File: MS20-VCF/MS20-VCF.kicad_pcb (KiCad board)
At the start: 2 copper layers, 127.5 x 133 mm, 112 parts, among them J1 Conn_CircuitBoard, J10 Conn_CircuitBoard, J11 Conn_JackBoard, J12 Conn_JackBoard, J13 FilterCV2, J14 FilterIn2, J15 FilterOut2, J2 Conn_CircuitBoard, J3 Conn_JackBoard, J4 Conn_JackBoard, J5 Power Input, J6 FilterCV1, J7 FilterIn1, J8 FilterOut1, J9 Conn_CircuitBoard, Q1 BC559, Q2 BC559, Q3 BC559, Q4 BC559, SW1 Hpass/Lpass Switch, SW2 Bandpass, SW3 Hpass/Lpass Switch, U1 LM13700, U2 TL072, U3 LM13700, U4 TL072

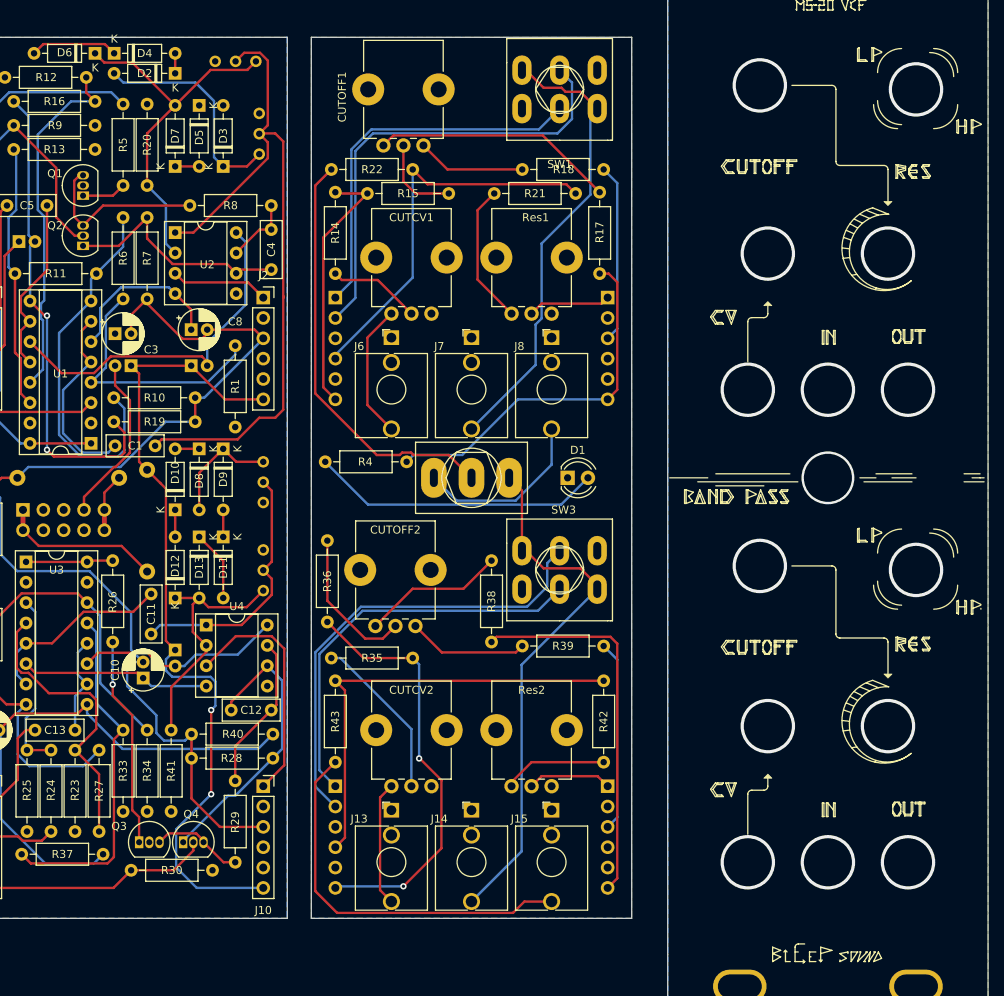
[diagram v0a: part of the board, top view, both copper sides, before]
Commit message: updgrade MS20
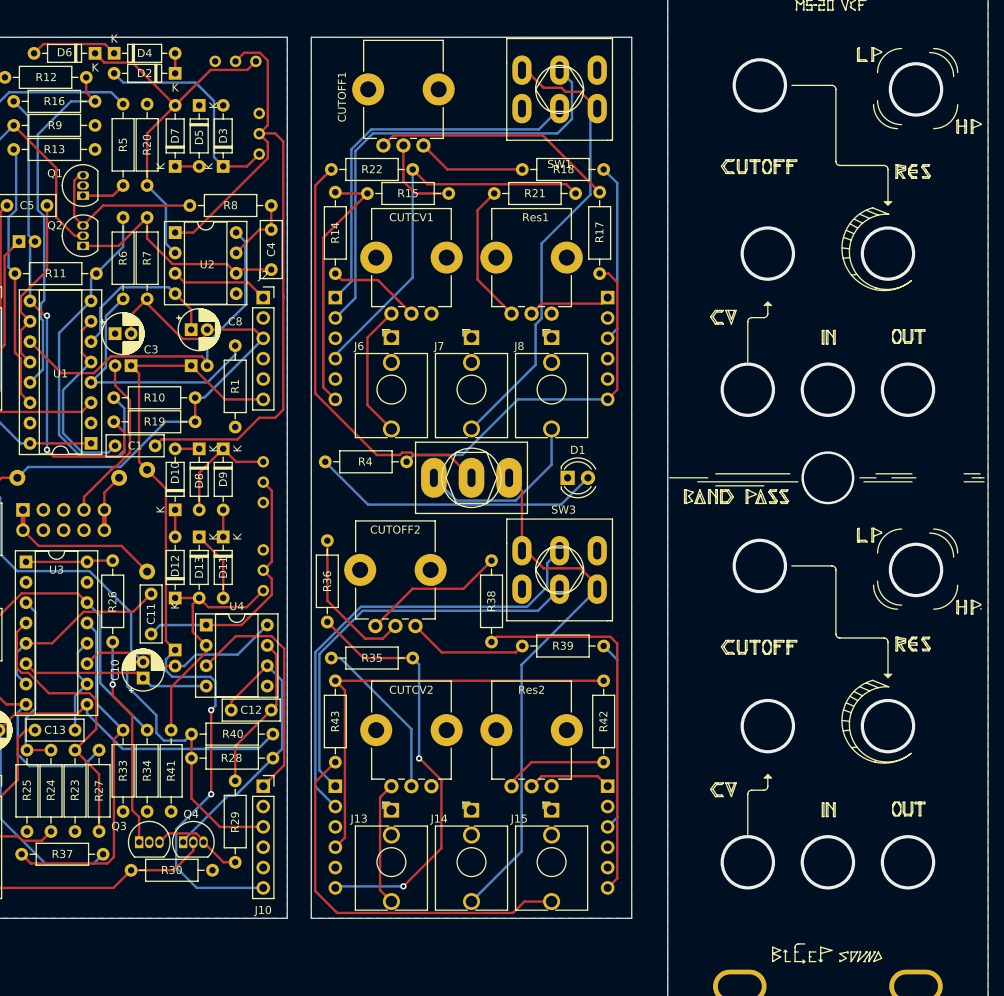
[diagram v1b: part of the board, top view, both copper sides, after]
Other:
- net class Default removed
- net class Power removed

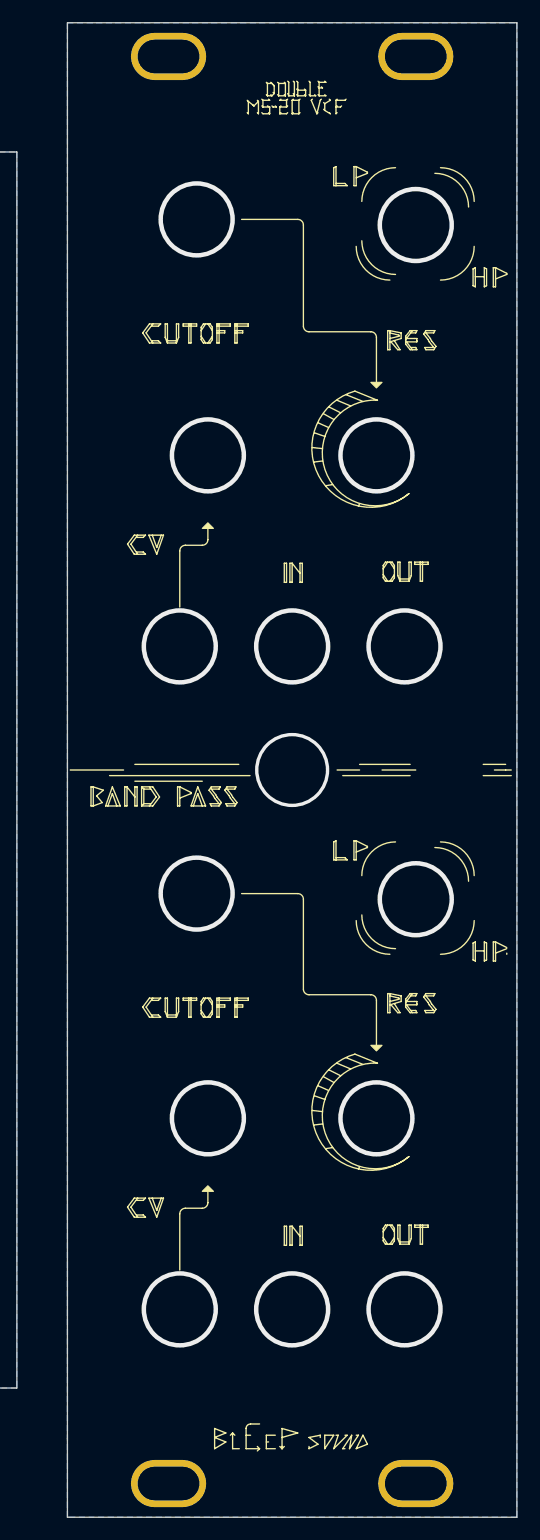
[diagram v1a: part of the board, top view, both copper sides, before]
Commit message: Update gerber MS20-VCF
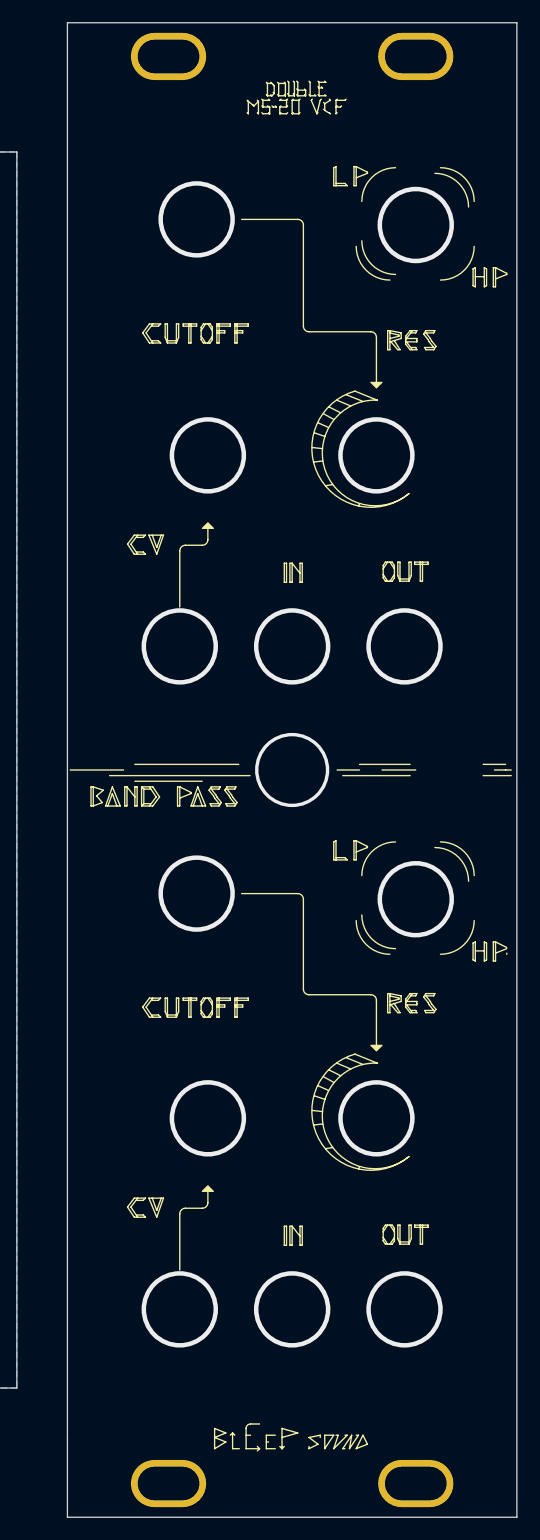
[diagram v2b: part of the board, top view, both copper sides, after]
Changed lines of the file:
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@@
     (fp_line (start 4 -2.75) (end -1.45 -2.75) (layer "F.CrtYd") (width 0.05))
     (fp_line (start -0.73 -1.32665) (end -0.73 1.32665) (layer "F.Fab") (width 0.1))
-    (fp_arc (start -0.73 -1.32665) (mid 3.67 0.000306) (end -0.730339 1.32614) (layer "F.Fab") (width 0.1))
+    (fp_arc (start -0.73 -1.32665) (mid 3.670001 0.000308) (end -0.730339 1.32614) (layer "F.Fab") (width 0.1))
     (fp_circle (center 1.27 0) (end 3.27 0) (layer "F.Fab") (width 0.1) (fill none))
     (pad "1" thru_hole rect locked (at 0 0) (size 1.8 1.8) (drill 0.9) (layers *.Cu *.Mask)
@@
   (gr_line (start 140.7 61) (end 139.8 60.6) (layer "F.SilkS") (width 0.12))
   (gr_arc (start 147.880994 66.91004) (mid 140.425465 64.78058) (end 145.085033 58.583166) (layer "F.SilkS") (width 0.12))
-  (gr_arc (start 147.9 66.9) (mid 139.860984 65.315822) (end 143.085033 57.783166) (layer "F.SilkS") (width 0.12))
+  (gr_arc (start 147.9 66.9) (mid 139.860985 65.315822) (end 143.085033 57.783166) (layer "F.SilkS") (width 0.12))
   (gr_line (start 143.8 58.7) (end 142.3 58.1) (layer "F.SilkS") (width 0.12))
   (gr_arc (start 130 71) (mid 129.853553 71.353553) (end 129.5 71.5) (layer "F.SilkS") (width 0.12))
@@
   (gr_line (start 141.2 119.3) (end 140.3 118.8) (layer "F.SilkS") (width 0.12))
   (gr_line (start 140.414967 120.816834) (end 139.5 120.5) (layer "F.SilkS") (width 0.12))
-  (gr_arc (start 147.9 125.9) (mid 139.860984 124.315822) (end 143.085033 116.783166) (layer "F.SilkS") (width 0.12))
+  (gr_arc (start 147.9 125.9) (mid 139.860985 124.315822) (end 143.085033 116.783166) (layer "F.SilkS") (width 0.12))
   (gr_line (start 140.2 121.9) (end 139.3 121.8) (layer "F.SilkS") (width 0.12))
   (gr_line (start 139.4 123.1) (end 140.2 123) (layer "F.SilkS") (width 0.12))
@@
   (gr_line (start 137.5 139.5) (end 137.5 133.7) (layer "Dwgs.User") (width 0.15))
   (gr_line (start 147.5 139.5) (end 147.5 133.5) (layer "Dwgs.User") (width 0.15))
-  (gr_line (start 129 42.5) (end 84.5 42.5) (layer "Dwgs.User") (width 0.15))
   (gr_line (start 113 95) (end 73 95) (layer "Dwgs.User") (width 0.15))
   (gr_line (start 69.999999 36.5) (end 70 146.5) (layer "Edge.Cuts") (width 0.05))
@@
   (segment (start 49.257997 67.700001) (end 46.650001 70.307997) (width 0.3) (layer "B.Cu") (net 15))
   (segment (start 54.202002 115) (end 52.552001 113.349999) (width 0.3) (layer "F.Cu") (net 16))
+  (segment (start 46.350001 113.349999) (end 45 114.7) (width 0.3) (layer "F.Cu") (net 16))
   (segment (start 52.552001 113.349999) (end 46.350001 113.349999) (width 0.3) (layer "F.Cu") (net 16))
   (segment (start 56 115) (end 54.202002 115) (width 0.3) (layer "F.Cu") (net 16))
-  (segment (start 46.350001 113.349999) (end 45 114.7) (width 0.3) (layer "F.Cu") (net 16))
   (segment (start 45.350001 114.349999) (end 45 114.7) (width 0.3) (layer "B.Cu") (net 16))
   (segment (start 63.809999 113.570001) (end 58.561369 113.570001) (width 0.3) (layer "B.Cu") (net 16))
@@
   (zone (net 1) (net_name "GND") (layer "B.Cu") (hatch edge 0.508)
     (connect_pads (clearance 0.508))
-    (min_thickness 0.254)
+    (min_thickness 0.254) (filled_areas_thickness no)
     (fill yes (thermal_gap 0.508) (thermal_bridge_width 0.508))
     (polygon
@@
   (zone (net 1) (net_name "GND") (layer "B.Cu") (hatch edge 0.508)
     (connect_pads (clearance 0.508))
-    (min_thickness 0.254)
+    (min_thickness 0.254) (filled_areas_thickness no)
     (fill yes (thermal_gap 0.508) (thermal_bridge_width 0.508))
     (polygon
@@
       )
     )
-  )
-  (zone (net 1) (net_name "GND") (layer "B.Cu") (hatch edge 0.508)
-    (connect_pads (clearance 0.508))
-    (min_thickness 0.254)
-    (fill yes (thermal_gap 0.508) (thermal_bridge_width 0.508))
-    (polygon
-      (pts
-        (xy 157.5 158)
-        (xy 117.5 158)
-        (xy 117.5 25)
-        (xy 157.5 25)
-      )
-    )

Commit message: update MS-20 VCF (increase size)
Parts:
- added C15: 0.1µ, Capacitor_THT:CP_Radial_D5.0mm_P2.00mm, F.Cu at (34.0, 107.5)
- added C16: 0.1µ, Capacitor_THT:CP_Radial_D5.0mm_P2.00mm, F.Cu at (34.0, 103.5)
- added C17: 0.1µ, Capacitor_THT:CP_Radial_D5.0mm_P2.00mm, F.Cu at (34.0, 91.5)
- added C18: 0.1µ, Capacitor_THT:CP_Radial_D5.0mm_P2.00mm, F.Cu at (37.0, 98.0)
- C2, C6, C7, C9: moved to F.Cu
- moved H2 79.5 mm to (228.0, 29.5)
- moved H3 79.5 mm to (228.0, 153.5)
- moved R4 64.5 mm to (147.0, 71.9), turned to -90 degrees
- moved H1 59.5 mm to (186.0, 29.5)
- moved H4 59.5 mm to (186.0, 153.5)
- moved R38 57.8 mm to (152.0, 113.9)
- moved R22 56.9 mm to (130.1, 69.0), turned to 180 degrees
- moved CUTOFF2 56.5 mm to (142.5, 110.0)
- moved CUTCV1 52.5 mm to (140.5, 71.0)
- moved J6 52.0 mm to (135.0, 74.0)
- moved D1 43.6 mm to (148.3, 86.5), turned to 180 degrees
- moved R9 43.0 mm to (74.1, 80.0)
- moved J12 42.0 mm to (152.0, 130.0)
- moved J4 42.0 mm to (152.0, 69.0)
- moved R39 40.2 mm to (148.0, 124.1), turned to 90 degrees
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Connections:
- C7 pad 2: Net-(C7-Pad2) -> Net-(U2-Pad8)
- J1 pad 3: Net-(J1-Pad3) -> unconnected-(J1-Pad3)
- J1 pad 5: Net-(J1-Pad5) -> unconnected-(J1-Pad5)
- J10 pad 2: Net-(J10-Pad2) -> unconnected-(J10-Pad2)
- J11 pad 3: Net-(J11-Pad3) -> unconnected-(J11-Pad3)
- J11 pad 5: Net-(J11-Pad5) -> unconnected-(J11-Pad5)
- J12 pad 2: Net-(J12-Pad2) -> unconnected-(J12-Pad2)
- J13 pad TN: Net-(J13-PadTN) -> unconnected-(J13-PadTN)
- J14 pad TN: Net-(J14-PadTN) -> unconnected-(J14-PadTN)
- J15 pad TN: Net-(J15-PadTN) -> unconnected-(J15-PadTN)
- J2 pad 2: Net-(J2-Pad2) -> unconnected-(J2-Pad2)
- J3 pad 3: Net-(J3-Pad3) -> unconnected-(J3-Pad3)
- J3 pad 5: Net-(J3-Pad5) -> unconnected-(J3-Pad5)
- J4 pad 2: Net-(J4-Pad2) -> unconnected-(J4-Pad2)
- J6 pad TN: Net-(J6-PadTN) -> unconnected-(J6-PadTN)
- J7 pad TN: Net-(J7-PadTN) -> unconnected-(J7-PadTN)
- J8 pad TN: Net-(J8-PadTN) -> unconnected-(J8-PadTN)
- J9 pad 3: Net-(J9-Pad3) -> unconnected-(J9-Pad3)
- J9 pad 5: Net-(J9-Pad5) -> unconnected-(J9-Pad5)
- SW1 pad 1: Net-(SW1-Pad1) -> unconnected-(SW1-Pad1)
- SW3 pad 1: Net-(SW3-Pad1) -> unconnected-(SW3-Pad1)
- U1 pad 11: Net-(C7-Pad2) -> Net-(U1-Pad11)
- U1 pad 15: Net-(U1-Pad15) -> unconnected-(U1-Pad15)
- U1 pad 2: Net-(U1-Pad2) -> unconnected-(U1-Pad2)
- U1 pad 6: Net-(C8-Pad1) -> Net-(C18-Pad1)
- U2 pad 8: Net-(C7-Pad2) -> Net-(U2-Pad8)
- U3 pad 11: Net-(C9-Pad2) -> Net-(C15-Pad2)
- U3 pad 15: Net-(U3-Pad15) -> unconnected-(U3-Pad15)
- U3 pad 2: Net-(U3-Pad2) -> unconnected-(U3-Pad2)
- U3 pad 6: Net-(C10-Pad1) -> Net-(C16-Pad1)
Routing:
- net Net-(R5-Pad2): track 71.7 -> 13.4 mm
- net Net-(C7-Pad2): track 44.5 -> 0.00 mm
- net /ResOut: track 22.6 -> 57.4 mm, vias 0 -> 1
- net -12V: track 183.6 -> 218.2 mm, vias 0 -> 1
- net Net-(C18-Pad1): track 0.00 -> 34.1 mm, vias 0 -> 1
- net Net-(C14-Pad2): track 66.0 -> 32.3 mm
- net Net-(C1-Pad2): track 88.4 -> 54.8 mm
- net Net-(D1-Pad2): track 36.4 -> 4.94 mm
- net Net-(R2-Pad2): track 45.7 -> 16.2 mm
- net Net-(CUTOFF2-Pad2): track 18.6 -> 47.4 mm
- net +12V: track 196.4 -> 225.1 mm, vias 2 -> 0
- net Net-(CUTCV1-Pad2): track 11.6 -> 38.5 mm
- net Net-(U1-Pad11): track 0.00 -> 23.3 mm
- net Net-(R10-Pad2): track 47.1 -> 24.2 mm
- net /FilterOut: track 52.9 -> 30.2 mm
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- added copper zone on F.Cu, net GND
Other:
- board size 127.5 x 133 mm -> 207 x 130 mm
- board text added: "12HP"
- board text added: "Double MS-20 VCF V1.0 BleepSound 2022"
- board text added: "board 1/2"
- board text added: "board 2/2"
- board text removed: "8HP"
